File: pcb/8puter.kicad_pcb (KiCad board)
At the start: 2 copper layers, 120 x 100 mm, 82 parts, among them J1 PWR-DC, U2 74AHC74, U3 SN74LVC1G14DBV, U6 MAX811MEUS-T, X1 ECS-2200BX-100, Y1 1.8432MHz

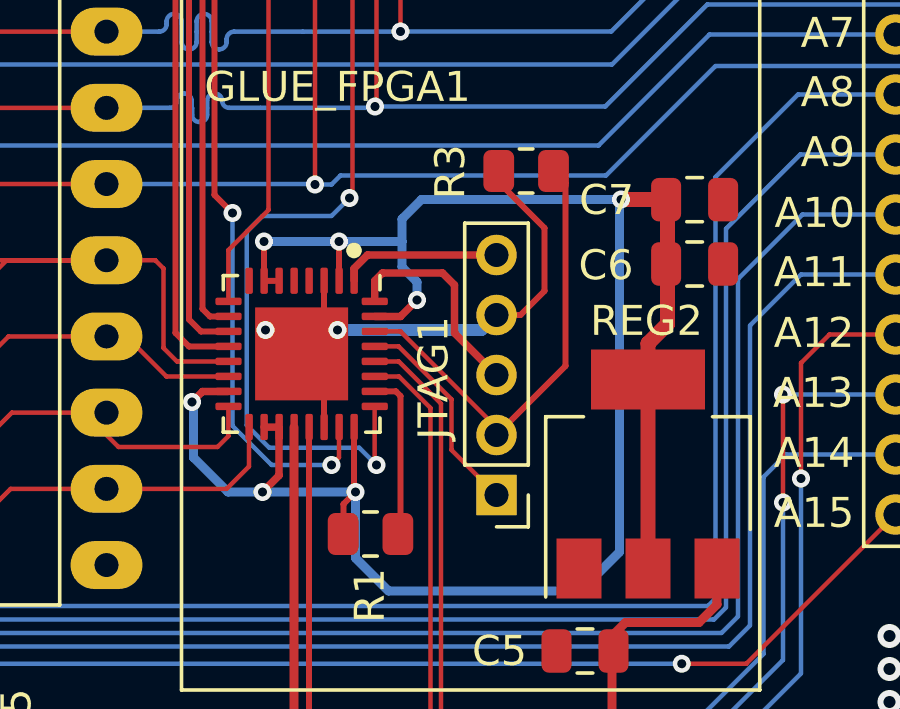
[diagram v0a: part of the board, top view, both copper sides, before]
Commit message: Gerber Plots
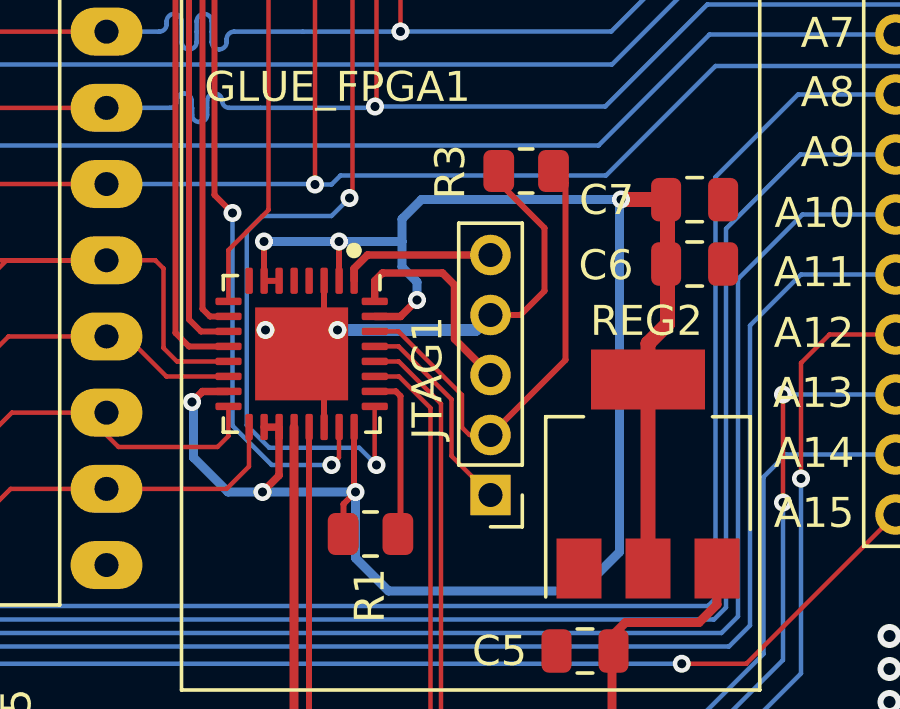
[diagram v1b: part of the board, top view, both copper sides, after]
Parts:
- moved JTAG1 0.20 mm to (184.4, 119.4)
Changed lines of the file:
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@@
   )
   (footprint "Connector_PinHeader_2.00mm:PinHeader_1x05_P2.00mm_Vertical" (layer "F.Cu")
-    (at 184.598 119.445 180)
+    (at 184.398 119.445 180)
     (descr "Through hole straight pin header, 1x05, 2.00mm pitch, single row")
     (tags "Through hole pin header THT 1x05 2.00mm single row")
@@
     (style (thickness 0.1) (arrow_length 1.27) (text_position_mode 0) (extension_height 0.58642) (extension_offset 0.5) keep_text_aligned)
   )
-  (segment (start 186.198 110.545) (end 186.198 112.645) (width 0.2) (layer "F.Cu") (net 1))
   (segment (start 167.898 58.395) (end 167.898 59.597162) (width 0.2) (layer "F.Cu") (net 1))
   (segment (start 105.398 52.245) (end 102.798 52.245) (width 0.5) (layer "F.Cu") (net 1))
   (segment (start 167.798489 60.193327) (end 168.150162 60.545) (width 0.2) (layer "F.Cu") (net 1))
-  (segment (start 185.398 113.445) (end 184.598 113.445) (width 0.2) (layer "F.Cu") (net 1))
   (segment (start 132.298 38.645) (end 125.498 38.645) (width 0.4) (layer "F.Cu") (net 1))
   (segment (start 101.298 53.745) (end 96.198 53.745) (width 0.5) (layer "F.Cu") (net 1))
   (segment (start 169.8105 51.9825) (end 172.49752 51.9825) (width 0.2) (layer "F.Cu") (net 1))
   (segment (start 164.543349 51.9825) (end 169.8105 51.9825) (width 0.2) (layer "F.Cu") (net 1))
+  (segment (start 184.673 109.02) (end 186.198 110.545) (width 0.2) (layer "F.Cu") (net 1))
   (segment (start 167.898 58.395) (end 167.898 55.245) (width 0.2) (layer "F.Cu") (net 1))
   (segment (start 98.063 70.53) (end 103.683 70.53) (width 0.4) (layer "F.Cu") (net 1))
@@
   (segment (start 193.023 54.995) (end 193.023 58.82) (width 0.3) (layer "F.Cu") (net 1))
   (segment (start 188.473 58.52) (end 189.098 59.145) (width 0.3) (layer "F.Cu") (net 1))
-  (segment (start 186.198 112.645) (end 185.398 113.445) (width 0.2) (layer "F.Cu") (net 1))
+  (segment (start 184.673 108.645) (end 184.673 109.02) (width 0.2) (layer "F.Cu") (net 1))
   (segment (start 191.073 54.995) (end 191.073 53.82) (width 0.3) (layer "F.Cu") (net 1))
   (segment (start 188.473 54.995) (end 188.473 58.52) (width 0.3) (layer "F.Cu") (net 1))
@@
   (segment (start 172.49752 51.94548) (end 172.898 51.545) (width 0.2) (layer "F.Cu") (net 1))
   (segment (start 102.798 52.245) (end 102.698 52.345) (width 0.5) (layer "F.Cu") (net 1))
+  (segment (start 186.198 112.645) (end 185.398 113.445) (width 0.2) (layer "F.Cu") (net 1))
   (segment (start 167.898 59.597162) (end 167.798489 59.696673) (width 0.2) (layer "F.Cu") (net 1))
   (segment (start 189.198 59.245) (end 190.348 59.245) (width 0.2) (layer "F.Cu") (net 1))
@@
   (segment (start 106.398 70.545) (end 103.798 70.545) (width 0.4) (layer "F.Cu") (net 1))
   (segment (start 103.798 70.545) (end 103.748 70.595) (width 0.4) (layer "F.Cu") (net 1))
+  (segment (start 186.198 110.545) (end 186.198 112.645) (width 0.2) (layer "F.Cu") (net 1))
   (segment (start 141.998 46.845) (end 142.498 46.345) (width 0.4) (layer "F.Cu") (net 1))
   (segment (start 178.848005 112.307488) (end 178.848005 113.994988) (width 0.2) (layer "F.Cu") (net 1))
-  (segment (start 184.673 109.02) (end 186.198 110.545) (width 0.2) (layer "F.Cu") (net 1))
   (segment (start 167.898 55.245) (end 167.6355 54.9825) (width 0.2) (layer "F.Cu") (net 1))
   (segment (start 141.648 46.845) (end 141.998 46.845) (width 0.4) (layer "F.Cu") (net 1))
@@
   (segment (start 167.798489 59.696673) (end 167.798489 60.193327) (width 0.2) (layer "F.Cu") (net 1))
   (segment (start 103.683 70.53) (end 103.748 70.595) (width 0.4) (layer "F.Cu") (net 1))
-  (segment (start 184.673 108.645) (end 184.673 109.02) (width 0.2) (layer "F.Cu") (net 1))
+  (segment (start 185.398 113.445) (end 184.398 113.445) (width 0.2) (layer "F.Cu") (net 1))
   (via (at 202.898 126.345) (size 0.8) (drill 0.4) (layers "F.Cu" "B.Cu") (net 1))
   (via (at 202.898 124.145) (size 0.8) (drill 0.4) (layers "F.Cu" "B.Cu") (net 1))
@@
   (segment (start 202.898 124.145) (end 197.698 124.145) (width 0.4) (layer "B.Cu") (net 1))
   (segment (start 176.898005 113.944988) (end 179.298005 113.944988) (width 0.4) (layer "B.Cu") (net 1))
-  (segment (start 179.298005 113.944988) (end 184.098012 113.944988) (width 0.4) (layer "B.Cu") (net 1))
   (segment (start 183.028 44.715) (end 196.168 44.715) (width 0.5) (layer "B.Cu") (net 1))
   (segment (start 172.898 52.845) (end 175.098 55.045) (width 0.2) (layer "B.Cu") (net 1))
@@
   (segment (start 136.698 52.945) (end 136.198 53.445) (width 0.25) (layer "B.Cu") (net 1))
   (segment (start 185.598 78.945) (end 191.298 78.945) (width 0.5) (layer "B.Cu") (net 1))
-  (segment (start 184.098012 113.944988) (end 184.598 113.445) (width 0.4) (layer "B.Cu") (net 1))
+  (segment (start 179.298005 113.944988) (end 183.898012 113.944988) (width 0.4) (layer "B.Cu") (net 1))
   (segment (start 172.898 51.545) (end 172.898 52.845) (width 0.2) (layer "B.Cu") (net 1))
   (segment (start 125.598 38.645) (end 125.598 41.345) (width 0.4) (layer "B.Cu") (net 1))
@@
   (segment (start 141.498 41.2945) (end 141.498 38.945) (width 0.4) (layer "B.Cu") (net 1))
   (segment (start 198.198 85.845) (end 198.198 86.345) (width 0.5) (layer "B.Cu") (net 1))
+  (segment (start 183.898012 113.944988) (end 184.398 113.445) (width 0.4) (layer "B.Cu") (net 1))
   (segment (start 130.298 53.445) (end 128.008 51.155) (width 0.25) (layer "B.Cu") (net 1))
   (segment (start 115.598 46.245) (end 118.298 46.245) (width 0.4) (layer "B.Cu") (net 1))
@@
   (segment (start 182.398 130.245) (end 182.373989 130.269011) (width 0.2) (layer "B.Cu") (net 58))
   (segment (start 97.422011 130.269011) (end 95.498 128.345) (width 0.2) (layer "B.Cu") (net 58))
+  (segment (start 179.852219 111.890781) (end 180.298 111.445) (width 0.25) (layer "F.Cu") (net 59))
   (segment (start 179.852219 112.303274) (end 179.852219 111.890781) (width 0.25) (layer "F.Cu") (net 59))
   (segment (start 180.298 111.445) (end 184.598 111.445) (width 0.25) (layer "F.Cu") (net 59))
-  (segment (start 179.852219 111.890781) (end 180.298 111.445) (width 0.25) (layer "F.Cu") (net 59))
   (segment (start 186.198005 71.894988) (end 186.198005 66.945005) (width 0.15) (layer "F.Cu") (net 60))
   (segment (start 186.198 66.345) (end 186.523 66.02) (width 0.15) (layer "F.Cu") (net 60))
@@
   (segment (start 181.398 120.6575) (end 181.3105 120.745) (width 0.2) (layer "F.Cu") (net 74))
   (segment (start 180.539719 115.990774) (end 181.243774 115.990774) (width 0.2) (layer "F.Cu") (net 74))
-  (segment (start 180.539719 114.490774) (end 181.332365 114.490774) (width 0.15) (layer "F.Cu") (net 75))
-  (segment (start 183.098 117.945) (end 184.598 119.445) (width 0.15) (layer "F.Cu") (net 75))
-  (segment (start 183.098 116.256409) (end 183.098 117.945) (width 0.15) (layer "F.Cu") (net 75))
+  (segment (start 183.098 116.256409) (end 183.098 118.145) (width 0.15) (layer "F.Cu") (net 75))
   (segment (start 181.332365 114.490774) (end 183.098 116.256409) (width 0.15) (layer "F.Cu") (net 75))
-  (segment (start 186.898 115.145) (end 184.598 117.445) (width 0.2) (layer "F.Cu") (net 76))
-  (segment (start 186.898 109.045) (end 186.898 115.145) (width 0.2) (layer "F.Cu") (net 76))
-  (segment (start 184.598 117.195) (end 184.598 117.445) (width 0.15) (layer "F.Cu") (net 76))
-  (segment (start 181.393774 113.990774) (end 184.598 117.195) (width 0.15) (layer "F.Cu") (net 76))
-  (segment (start 180.539719 113.990774) (end 181.393774 113.990774) (width 0.15) (layer "F.Cu") (net 76))
+  (segment (start 183.098 118.145) (end 184.398 119.445) (width 0.15) (layer "F.Cu") (net 75))
+  (segment (start 180.539719 114.490774) (end 181.332365 114.490774) (width 0.15) (layer "F.Cu") (net 75))
   (segment (start 186.498 108.645) (end 186.898 109.045) (width 0.2) (layer "F.Cu") (net 76))
-  (segment (start 183.198 114.045) (end 184.598 115.445) (width 0.25) (layer "F.Cu") (net 77))
-  (segment (start 183.198 112.445) (end 183.198 114.045) (width 0.25) (layer "F.Cu") (net 77))
-  (segment (start 182.798 112.045) (end 183.198 112.445) (width 0.25) (layer "F.Cu") (net 77))
+  (segment (start 180.539719 113.990774) (end 181.32666 113.990774) (width 0.15) (layer "F.Cu") (net 76))
+  (segment (start 186.898 114.945) (end 184.398 117.445) (width 0.2) (layer "F.Cu") (net 76))
+  (segment (start 181.32666 113.990774) (end 183.44752 116.111634) (width 0.15) (layer "F.Cu") (net 76))
+  (segment (start 183.698 117.445) (end 184.398 117.445) (width 0.15) (layer "F.Cu") (net 76))
+  (segment (start 186.898 109.045) (end 186.898 114.945) (width 0.2) (layer "F.Cu") (net 76))
+  (segment (start 183.44752 116.111634) (end 183.44752 117.19452) (width 0.15) (layer "F.Cu") (net 76))
+  (segment (start 183.44752 117.19452) (end 183.698 117.445) (width 0.15) (layer "F.Cu") (net 76))
   (segment (start 180.539719 112.303281) (end 180.798 112.045) (width 0.25) (layer "F.Cu") (net 77))
+  (segment (start 182.798 112.045) (end 183.198 112.445) (width 0.25) (layer "F.Cu") (net 77))
   (segment (start 180.539719 112.990774) (end 180.539719 112.303281) (width 0.25) (layer "F.Cu") (net 77))
+  (segment (start 183.198 112.445) (end 183.198 114.245) (width 0.25) (layer "F.Cu") (net 77))
   (segment (start 180.798 112.045) (end 182.798 112.045) (width 0.25) (layer "F.Cu") (net 77))
+  (segment (start 183.198 114.245) (end 184.398 115.445) (width 0.25) (layer "F.Cu") (net 77))
   (segment (start 143.198 51.245) (end 143.198 53.3075) (width 0.25) (layer "F.Cu") (net 89))
   (segment (start 143.198 53.3075) (end 143.1605 53.345) (width 0.25) (layer "F.Cu") (net 89))
